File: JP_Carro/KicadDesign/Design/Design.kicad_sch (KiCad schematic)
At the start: 14 parts, among them J10 Puente_H2, J11 A MOTOR, J12 B MOTOR, J13 SENSOR_SOURCE, J5 SENSOR, J6 Conn_01x20_Socket, J7 Conn_01x20_Socket, J8 Puente H, J9 9V, U3.3V1 LM317_TO-220

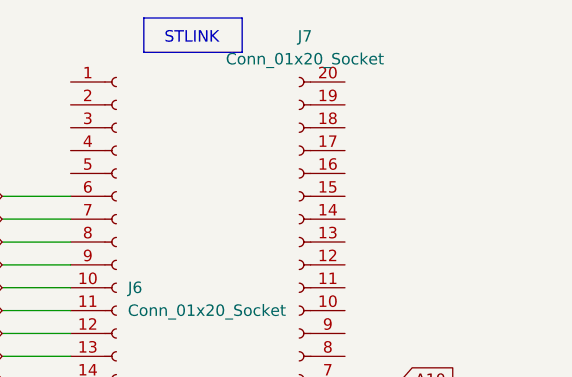
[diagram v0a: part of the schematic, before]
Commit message: Placa terminada
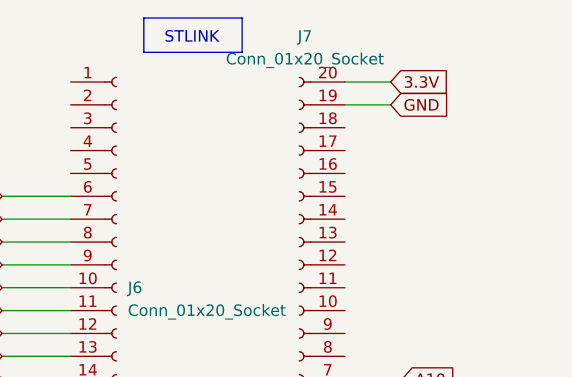
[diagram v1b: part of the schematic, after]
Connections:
- net 3.3V: now also J7.20 (Pin_20)
- net GND: now also J7.19 (Pin_19)
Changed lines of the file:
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@@
 	(wire
 		(pts
+			(xy 200.66 62.23) (xy 207.01 62.23)
+		)
+		(stroke
+			(width 0)
+			(type default)
+		)
+	)
+	(wire
+		(pts
 			(xy 107.95 104.14) (xy 107.95 101.6)
 		)
@@
 	(wire
 		(pts
+			(xy 237.49 21.59) (xy 242.57 21.59)
+		)
+		(stroke
+			(width 0)
+			(type default)
+		)
+	)
+	(wire
+		(pts
 			(xy 92.71 125.73) (xy 92.71 121.92)
 		)
@@
 	(wire
 		(pts
+			(xy 237.49 19.05) (xy 242.57 19.05)
+		)
+		(stroke
+			(width 0)
+			(type default)
+		)
+	)
+	(wire
+		(pts
 			(xy 77.47 104.14) (xy 77.47 125.73)
 		)
@@
 	(wire
 		(pts
-			(xy 200.66 62.23) (xy 207.01 62.23)
-		)
-		(stroke
-			(width 0)
-			(type default)
-		)
-	)
-	(wire
-		(pts
 			(xy 199.39 34.29) (xy 207.01 34.29)
 		)
@@
 		)
 	)
+	(global_label "3.3V"
+		(shape input)
+		(at 200.66 62.23 180)
+		(fields_autoplaced yes)
+		(effects
+			(font
+				(size 1.27 1.27)
+			)
+			(justify right)
+		)
+		(property "Intersheetrefs" "${INTERSHEET_REFS}"
+			(at 193.5624 62.23 0)
+			(hide yes)
+			(show_name no)
+			(do_not_autoplace no)
+			(effects
+				(font
+					(size 1.27 1.27)
+				)
+				(justify right)
+			)
+		)
+	)
 	(global_label "A2 AIN1"
 		(shape input)
@@
 		)
 	)
+	(global_label "3.3V"
+		(shape input)
+		(at 242.57 19.05 0)
+		(fields_autoplaced yes)
+		(effects
+			(font
+				(size 1.27 1.27)
+			)
+			(justify left)
+		)
+		(property "Intersheetrefs" "${INTERSHEET_REFS}"
+			(at 249.6676 19.05 0)
+			(hide yes)
+			(show_name no)
+			(do_not_autoplace no)
+			(effects
+				(font
+					(size 1.27 1.27)
+				)
+				(justify left)
+			)
+		)
+	)
 	(global_label "A5 BIN2"
 		(shape input)
@@
 	(global_label "3.3V"
 		(shape input)
-		(at 200.66 62.23 180)
-		(fields_autoplaced yes)
-		(effects
-			(font
-				(size 1.27 1.27)
-			)
-			(justify right)
-		)
-		(property "Intersheetrefs" "${INTERSHEET_REFS}"
-			(at 193.5624 62.23 0)
-			(hide yes)
-			(show_name no)
-			(do_not_autoplace no)
-			(effects
-				(font
-					(size 1.27 1.27)
-				)
-				(justify right)
-			)
-		)
-	)
-	(global_label "3.3V"
-		(shape input)
 		(at 124.46 49.53 180)
 		(fields_autoplaced yes)
@@
 			)
 		)
+	)
+	(global_label "GND"
+		(shape input)
+		(at 242.57 21.59 0)
+		(fields_autoplaced yes)
+		(effects
+			(font
+				(size 1.27 1.27)
+			)
+			(justify left)
+		)
+		(property "Intersheetrefs" "${INTERSHEET_REFS}"
+			(at 249.4257 21.59 0)
+			(hide yes)
+			(show_name no)
+			(do_not_autoplace no)
+			(effects
+				(font
+					(size 1.27 1.27)
+				)
+				(justify left)
+			)
+		)
